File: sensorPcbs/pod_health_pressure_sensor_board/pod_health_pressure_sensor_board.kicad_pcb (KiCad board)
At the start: 2 copper layers, 35.6 x 19 mm, 2 parts, among them J1 RJ45, U1 bmp180

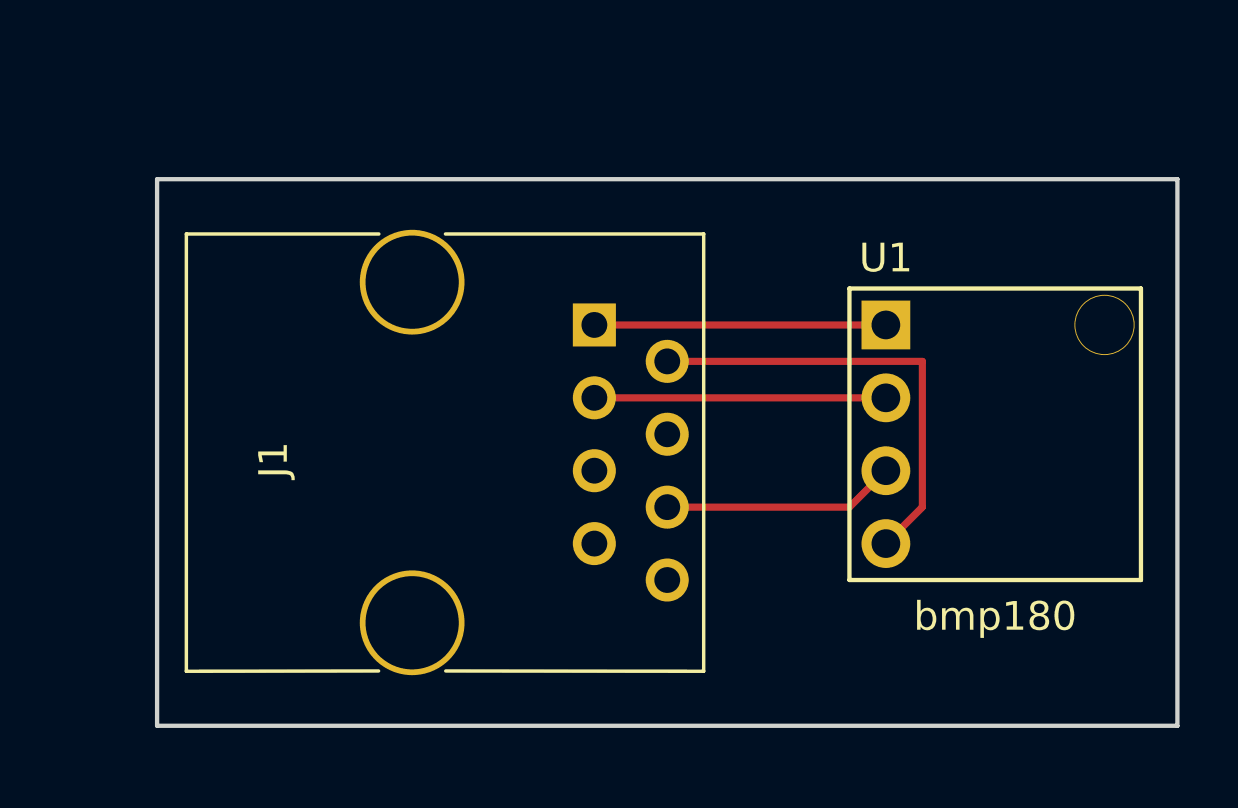
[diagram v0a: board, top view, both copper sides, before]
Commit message: added all the ferkin new ethernet shields to the sensor pcbs
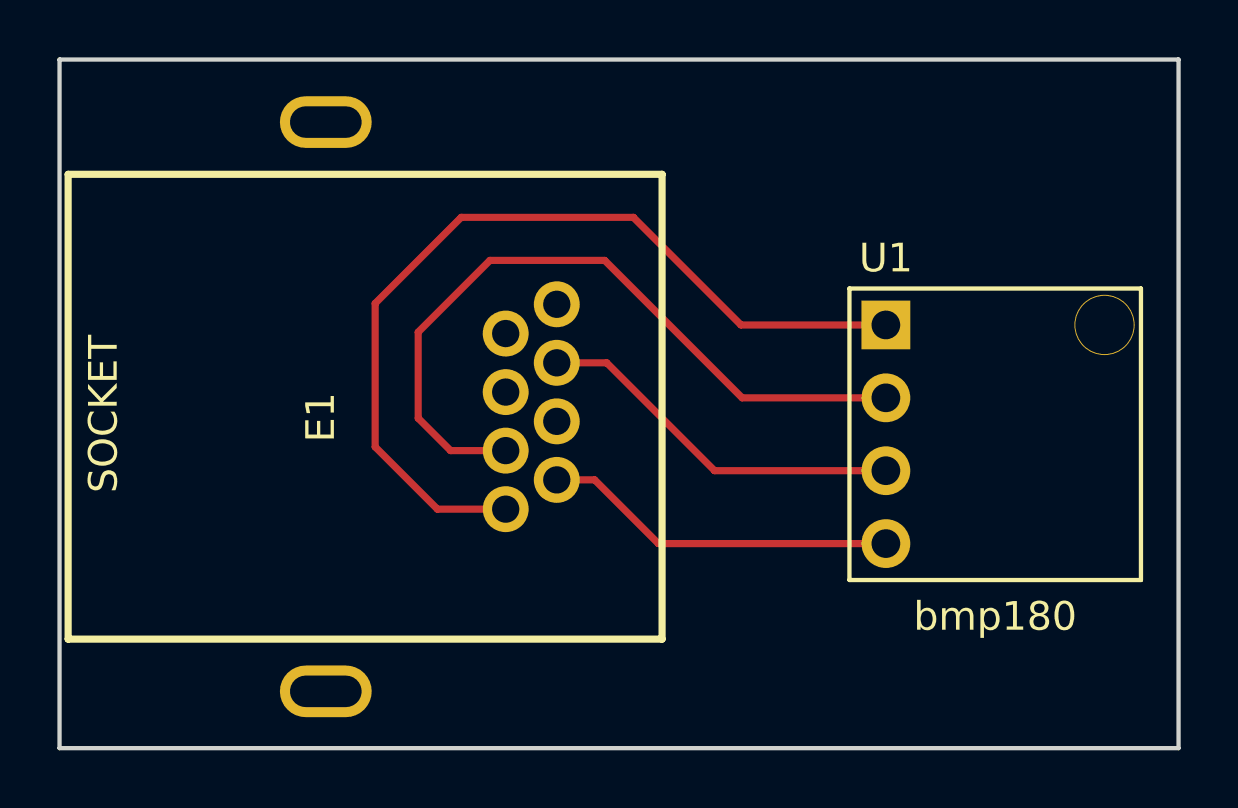
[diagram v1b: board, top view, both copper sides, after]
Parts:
- removed J1: RJ45, Connectors:RJ45_8
- added E1: RJE71-188-1401-ND, footprints:RJE71-188-1401-ND, F.Cu at (170.0, 90.0)
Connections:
- U1 pad 1: Net-(J1-Pad1) -> vin
- U1 pad 2: Net-(J1-Pad3) -> scl
- U1 pad 3: Net-(J1-Pad6) -> sda
- U1 pad 4: Net-(J1-Pad2) -> gnd
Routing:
- net vin: track 0.00 -> 31.0 mm
- net scl: track 0.00 -> 25.8 mm
- net Net-(J1-Pad2): track 15.8 -> 0.00 mm
- net sda: track 0.00 -> 13.0 mm
- net gnd: track 0.00 -> 12.4 mm
- net Net-(J1-Pad3): track 10.2 -> 0.00 mm
- net Net-(J1-Pad1): track 10.2 -> 0.00 mm
- net Net-(J1-Pad6): track 8.15 -> 0.00 mm
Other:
- board size 35.6 x 19 mm -> 39 x 24 mm
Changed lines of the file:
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@@
     (links 4)
     (no_connects 0)
-    (area 134.544999 87.554999 188.035001 111.835001)
+    (area 0 0 0 0)
     (thickness 1.6)
     (drawings 4)
-    (tracks 7)
+    (tracks 20)
     (zones 0)
     (modules 2)
@@
   )
   (net 0 "")
-  (net 1 "Net-(J1-Pad1)")
-  (net 2 "Net-(J1-Pad2)")
-  (net 3 "Net-(J1-Pad3)")
-  (net 4 "Net-(J1-Pad4)")
-  (net 5 "Net-(J1-Pad5)")
-  (net 6 "Net-(J1-Pad6)")
-  (net 7 "Net-(J1-Pad7)")
-  (net 8 "Net-(J1-Pad8)")
+  (net 1 vin)
+  (net 2 gnd)
+  (net 3 scl)
+  (net 4 "Net-(E1-Pad4)")
+  (net 5 "Net-(E1-Pad5)")
+  (net 6 sda)
+  (net 7 "Net-(E1-Pad8)")
+  (net 8 "Net-(E1-Pad7)")
   (net_class Default "This is the default net class."
     (clearance 0.2)
@@
     (uvia_dia 0.3)
     (uvia_drill 0.1)
-    (add_net "Net-(J1-Pad1)")
-    (add_net "Net-(J1-Pad2)")
-    (add_net "Net-(J1-Pad3)")
-    (add_net "Net-(J1-Pad4)")
-    (add_net "Net-(J1-Pad5)")
-    (add_net "Net-(J1-Pad6)")
-    (add_net "Net-(J1-Pad7)")
-    (add_net "Net-(J1-Pad8)")
-  )
-  (module Connectors:RJ45_8 (layer F.Cu)
-    (at 167.64 95.25 270)
-    (tags RJ45)
-    (fp_text reference J1 (at 4.7 11.18 270) (layer F.SilkS)
-      (effects (font (size 1 1) (thickness 0.15)))
-    )
-    (fp_text value RJ45 (at 4.59 6.25 270) (layer F.Fab)
-      (effects (font (size 1 1) (thickness 0.15)))
-    )
-    (fp_line (start -3.17 14.22) (end 12.07 14.22) (layer F.SilkS) (width 0.12))
-    (fp_line (start 12.07 -3.81) (end 12.06 5.18) (layer F.SilkS) (width 0.12))
-    (fp_line (start 12.07 -3.81) (end -3.17 -3.81) (layer F.SilkS) (width 0.12))
-    (fp_line (start -3.17 -3.81) (end -3.17 5.19) (layer F.SilkS) (width 0.12))
-    (fp_line (start 12.06 7.52) (end 12.07 14.22) (layer F.SilkS) (width 0.12))
-    (fp_line (start -3.17 7.51) (end -3.17 14.22) (layer F.SilkS) (width 0.12))
-    (fp_line (start -3.56 -4.06) (end 12.46 -4.06) (layer F.CrtYd) (width 0.05))
-    (fp_line (start -3.56 -4.06) (end -3.56 14.47) (layer F.CrtYd) (width 0.05))
-    (fp_line (start 12.46 14.47) (end 12.46 -4.06) (layer F.CrtYd) (width 0.05))
-    (fp_line (start 12.46 14.47) (end -3.56 14.47) (layer F.CrtYd) (width 0.05))
-    (pad Hole np_thru_hole circle (at 10.38 6.35 270) (size 3.65 3.65) (drill 3.25) (layers *.Cu *.SilkS *.Mask))
-    (pad Hole np_thru_hole circle (at -1.49 6.35 270) (size 3.65 3.65) (drill 3.25) (layers *.Cu *.SilkS *.Mask))
-    (pad 1 thru_hole rect (at 0 0 270) (size 1.5 1.5) (drill 0.9) (layers *.Cu *.Mask)
-      (net 1 "Net-(J1-Pad1)"))
-    (pad 2 thru_hole circle (at 1.27 -2.54 270) (size 1.5 1.5) (drill 0.9) (layers *.Cu *.Mask)
-      (net 2 "Net-(J1-Pad2)"))
-    (pad 3 thru_hole circle (at 2.54 0 270) (size 1.5 1.5) (drill 0.9) (layers *.Cu *.Mask)
-      (net 3 "Net-(J1-Pad3)"))
-    (pad 4 thru_hole circle (at 3.81 -2.54 270) (size 1.5 1.5) (drill 0.9) (layers *.Cu *.Mask)
-      (net 4 "Net-(J1-Pad4)"))
-    (pad 5 thru_hole circle (at 5.08 0 270) (size 1.5 1.5) (drill 0.9) (layers *.Cu *.Mask)
-      (net 5 "Net-(J1-Pad5)"))
-    (pad 6 thru_hole circle (at 6.35 -2.54 270) (size 1.5 1.5) (drill 0.9) (layers *.Cu *.Mask)
-      (net 6 "Net-(J1-Pad6)"))
-    (pad 7 thru_hole circle (at 7.62 0 270) (size 1.5 1.5) (drill 0.9) (layers *.Cu *.Mask)
-      (net 7 "Net-(J1-Pad7)"))
-    (pad 8 thru_hole circle (at 8.89 -2.54 270) (size 1.5 1.5) (drill 0.9) (layers *.Cu *.Mask)
-      (net 8 "Net-(J1-Pad8)"))
-    (model Connectors.3dshapes/RJ45_8.wrl
-      (at (xyz 0.18 -0.25 0))
-      (scale (xyz 0.4 0.4 0.4))
-      (rotate (xyz 0 0 0))
-    )
+    (add_net "Net-(E1-Pad4)")
+    (add_net "Net-(E1-Pad5)")
+    (add_net "Net-(E1-Pad7)")
+    (add_net "Net-(E1-Pad8)")
+    (add_net gnd)
+    (add_net scl)
+    (add_net sda)
+    (add_net vin)
   )
   (module bmp180_footprints:bmp180 (layer F.Cu)
@@
     )
     (pad 1 thru_hole rect (at 0 0) (size 1.7 1.7) (drill 1) (layers *.Cu *.Mask)
-      (net 1 "Net-(J1-Pad1)"))
+      (net 1 vin))
     (pad 2 thru_hole oval (at 0 2.54) (size 1.7 1.7) (drill 1) (layers *.Cu *.Mask)
-      (net 3 "Net-(J1-Pad3)"))
+      (net 3 scl))
     (pad 3 thru_hole oval (at 0 5.08) (size 1.7 1.7) (drill 1) (layers *.Cu *.Mask)
-      (net 6 "Net-(J1-Pad6)"))
+      (net 6 sda))
     (pad 4 thru_hole oval (at 0 7.62) (size 1.7 1.7) (drill 1) (layers *.Cu *.Mask)
-      (net 2 "Net-(J1-Pad2)"))
+      (net 2 gnd))
     (pad "" np_thru_hole circle (at 7.62 0) (size 2.1 2.1) (drill 2.032) (layers *.Cu))
     (model ${KISYS3DMOD}/Socket_Strips.3dshapes/Socket_Strip_Straight_1x04_Pitch2.54mm.wrl
@@
     )
   )
-  (gr_line (start 187.96 90.17) (end 152.4 90.17) (angle 90) (layer Edge.Cuts) (width 0.15))
-  (gr_line (start 187.96 109.22) (end 187.96 90.17) (angle 90) (layer Edge.Cuts) (width 0.15))
-  (gr_line (start 152.4 109.22) (end 187.96 109.22) (angle 90) (layer Edge.Cuts) (width 0.15))
-  (gr_line (start 152.4 90.17) (end 152.4 109.22) (angle 90) (layer Edge.Cuts) (width 0.15))
-  (segment (start 167.64 95.25) (end 177.8 95.25) (width 0.25) (layer F.Cu) (net 1) (status C00000))
-  (segment (start 170.18 96.52) (end 179.07 96.52) (width 0.25) (layer F.Cu) (net 2) (status 400000))
-  (segment (start 179.07 101.6) (end 177.8 102.87) (width 0.25) (layer F.Cu) (net 2) (status 800000))
-  (segment (start 179.07 96.52) (end 179.07 101.6) (width 0.25) (layer F.Cu) (net 2))
-  (segment (start 167.64 97.79) (end 177.8 97.79) (width 0.25) (layer F.Cu) (net 3) (status C00000))
-  (segment (start 170.18 101.6) (end 176.53 101.6) (width 0.25) (layer F.Cu) (net 6) (status 400000))
-  (segment (start 176.53 101.6) (end 177.8 100.33) (width 0.25) (layer F.Cu) (net 6) (status 800000))
+  (module footprints:RJE71-188-1401-ND (layer F.Cu)
+    (at 170 90 270)
+    (fp_text reference E1 (at 8.47 11.9 270) (layer F.SilkS)
+      (effects (font (size 1 1) (thickness 0.15)))
+    )
+    (fp_text value RJE71-188-1401-ND (at 14.5 11.39 360) (layer F.Fab)
+      (effects (font (size 1 1) (thickness 0.15)))
+    )
+    (fp_text user SOCKET (at 8.35 19.47 270) (layer F.SilkS)
+      (effects (font (size 1 1) (thickness 0.15)))
+    )
+    (fp_line (start 16.2 0) (end 16.2 20.7) (layer F.SilkS) (width 0.25))
+    (fp_line (start 0 20.7) (end 16.2 20.7) (layer F.SilkS) (width 0.25))
+    (fp_line (start 0 0) (end 16.2 0) (layer F.SilkS) (width 0.25))
+    (fp_line (start 0 0) (end 0 20.7) (layer F.SilkS) (width 0.25))
+    (pad 1 thru_hole circle (at 11.67 5.45 270) (size 1.6 1.6) (drill 0.95) (layers *.Cu *.Mask)
+      (net 1 vin))
+    (pad 2 thru_hole circle (at 10.65 3.67 270) (size 1.6 1.6) (drill 0.95) (layers *.Cu *.Mask)
+      (net 2 gnd))
+    (pad 3 thru_hole circle (at 9.63 5.45 270) (size 1.6 1.6) (drill 0.95) (layers *.Cu *.Mask)
+      (net 3 scl))
+    (pad 4 thru_hole circle (at 8.61 3.67 270) (size 1.6 1.6) (drill 0.95) (layers *.Cu *.Mask)
+      (net 4 "Net-(E1-Pad4)"))
+    (pad 5 thru_hole circle (at 7.59 5.45 270) (size 1.6 1.6) (drill 0.95) (layers *.Cu *.Mask)
+      (net 5 "Net-(E1-Pad5)"))
+    (pad 6 thru_hole circle (at 6.57 3.67 270) (size 1.6 1.6) (drill 0.95) (layers *.Cu *.Mask)
+      (net 6 sda))
+    (pad "" thru_hole oval (at -1.82 11.72 270) (size 1.8 3.2) (drill oval 1.1 2.5) (layers *.Cu *.Mask))
+    (pad "" thru_hole oval (at 18.02 11.72 270) (size 1.8 3.2) (drill oval 1.1 2.5) (layers *.Cu *.Mask))
+    (pad 8 thru_hole circle (at 4.53 3.67 270) (size 1.6 1.6) (drill 0.95) (layers *.Cu *.Mask)
+      (net 7 "Net-(E1-Pad8)"))
+    (pad 7 thru_hole circle (at 5.55 5.45 270) (size 1.6 1.6) (drill 0.95) (layers *.Cu *.Mask)
+      (net 8 "Net-(E1-Pad7)"))
+  )
+  (gr_line (start 149 86) (end 149 110) (angle 90) (layer Edge.Cuts) (width 0.15))
+  (gr_line (start 188 86) (end 149 86) (angle 90) (layer Edge.Cuts) (width 0.15))
+  (gr_line (start 188 110) (end 188 86) (angle 90) (layer Edge.Cuts) (width 0.15))
+  (gr_line (start 149 110) (end 188 110) (angle 90) (layer Edge.Cuts) (width 0.15))
+  (segment (start 164.55 101.67) (end 162.17 101.67) (width 0.25) (layer F.Cu) (net 1) (status 400000))
+  (segment (start 172.75 95.25) (end 177.8 95.25) (width 0.25) (layer F.Cu) (net 1) (status 800000))
+  (segment (start 169 91.5) (end 172.75 95.25) (width 0.25) (layer F.Cu) (net 1))
+  (segment (start 163 91.5) (end 169 91.5) (width 0.25) (layer F.Cu) (net 1))
+  (segment (start 160 94.5) (end 163 91.5) (width 0.25) (layer F.Cu) (net 1))
+  (segment (start 160 99.5) (end 160 94.5) (width 0.25) (layer F.Cu) (net 1))
+  (segment (start 162.17 101.67) (end 160 99.5) (width 0.25) (layer F.Cu) (net 1))
+  (segment (start 166.33 100.65) (end 167.65 100.65) (width 0.25) (layer F.Cu) (net 2) (status 400000))
+  (segment (start 169.87 102.87) (end 177.8 102.87) (width 0.25) (layer F.Cu) (net 2) (status 800000))
+  (segment (start 167.65 100.65) (end 169.87 102.87) (width 0.25) (layer F.Cu) (net 2))
+  (segment (start 164.55 99.63) (end 162.63 99.63) (width 0.25) (layer F.Cu) (net 3) (status 400000))
+  (segment (start 172.79 97.79) (end 177.8 97.79) (width 0.25) (layer F.Cu) (net 3) (status 800000))
+  (segment (start 168 93) (end 172.79 97.79) (width 0.25) (layer F.Cu) (net 3))
+  (segment (start 164 93) (end 168 93) (width 0.25) (layer F.Cu) (net 3))
+  (segment (start 161.5 95.5) (end 164 93) (width 0.25) (layer F.Cu) (net 3))
+  (segment (start 161.5 98.5) (end 161.5 95.5) (width 0.25) (layer F.Cu) (net 3))
+  (segment (start 162.63 99.63) (end 161.5 98.5) (width 0.25) (layer F.Cu) (net 3))
+  (segment (start 166.33 96.57) (end 168.07 96.57) (width 0.25) (layer F.Cu) (net 6) (status 400000))
+  (segment (start 171.83 100.33) (end 177.8 100.33) (width 0.25) (layer F.Cu) (net 6) (status 800000))
+  (segment (start 168.07 96.57) (end 171.83 100.33) (width 0.25) (layer F.Cu) (net 6))
 )
